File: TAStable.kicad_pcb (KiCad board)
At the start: 2 copper layers, 26.8 x 16.5 mm, 18 parts, among them J1 Conn_01x06_Pin, J2 ICSP, U1 74HCT1G04, U2 CS2300-CP, U3 74LVC1G14, U4 PIC16LF15313, U6 AZ1117-3.3

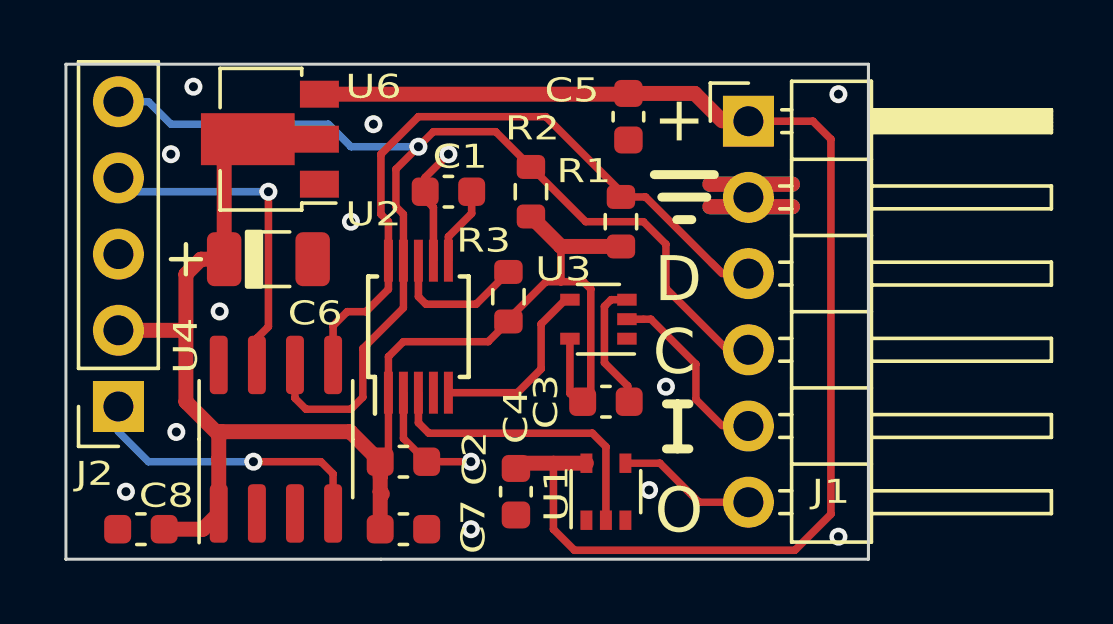
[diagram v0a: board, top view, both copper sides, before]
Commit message: more pics + cleanups
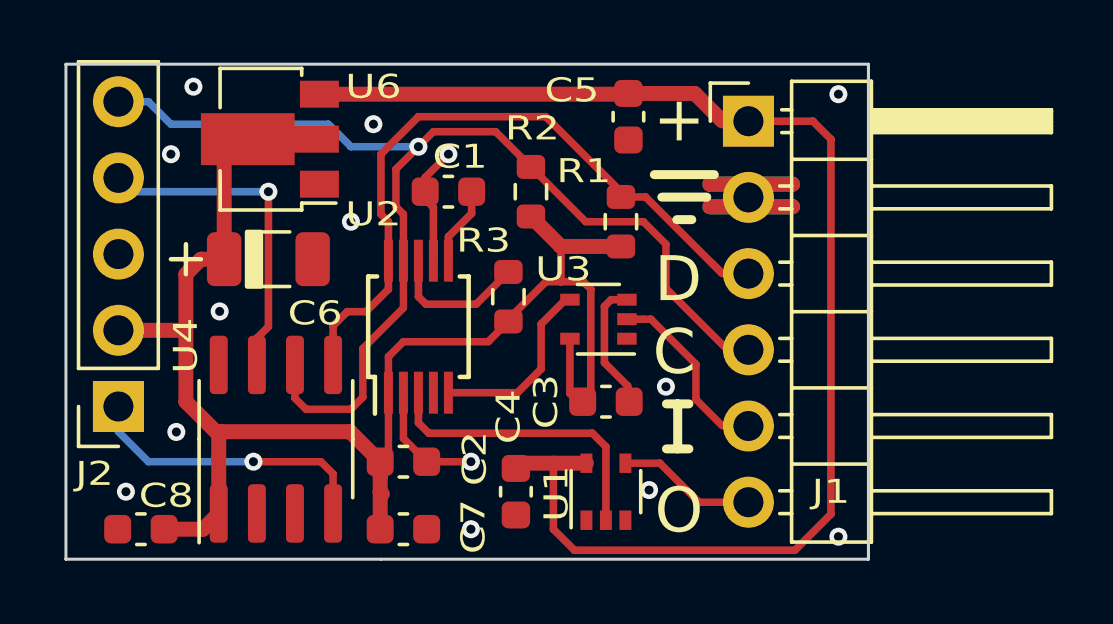
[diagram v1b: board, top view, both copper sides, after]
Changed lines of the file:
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@@
     (property "ki_keywords" "cap capacitor")
     (attr smd)
-    (fp_text reference "C4" (at -2.5 0 90) (layer "F.SilkS")
+    (fp_text reference "C4" (at -2.5 0.25 90) (layer "F.SilkS")
         (effects (font (size 0.8 1) (thickness 0.15)))
     )

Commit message: schematic
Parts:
- J1: value Conn_01x06_Pin -> IN/OUT
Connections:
- net Net-(J1-Pin_6) renamed /24MHz_OUT
- J1 pad 3: /I2C_SCL -> /I2C_SDA
- R1 pad 2: /I2C_SCL -> /I2C_SDA
- U2 pad 10: /I2C_SCL -> /I2C_SDA
- U4 pad 5: /I2C_SCL -> /I2C_SDA
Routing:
- net /I2C_SCL: track 61.8 -> 38.7 mm
- net /I2C_SDA: track 0.00 -> 23.1 mm
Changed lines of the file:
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@@
   (net 8 "/21MHz_IN")
   (net 9 "/I2C_SCL")
-  (net 10 "Net-(J1-Pin_6)")
+  (net 10 "/I2C_SDA")
   (net 11 "unconnected-(U4-RA5-Pad2)")
   (net 12 "unconnected-(U4-RA4-Pad3)")
@@
   (net 14 "/MCLR")
   (net 15 "/ICSPDAT")
+  (net 16 "/24MHz_OUT")
   (footprint "Package_SO:MSOP-10_3x3mm_P0.5mm" (layer "F.Cu")
     (at 130.25 100.5 90)
@@
       (net 9 "/I2C_SCL") (pinfunction "SCL/CCLK") (pintype "input"))
     (pad "10" smd rect (at 2.2 -1 90) (size 1.4 0.3) (layers "F.Cu" "F.Paste" "F.Mask")
-      (net 9 "/I2C_SCL") (pinfunction "SDA/CDIN") (pintype "bidirectional"))
+      (net 10 "/I2C_SDA") (pinfunction "SDA/CDIN") (pintype "bidirectional"))
     (model "${KICAD6_3DMODEL_DIR}/Package_SO.3dshapes/MSOP-10_3x3mm_P0.5mm.wrl"
       (offset (xyz 0 0 0))
@@
         (effects (font (size 0.8 1) (thickness 0.15)))
     )
-    (fp_text value "Conn_01x06_Pin" (at 1.865 16.18) (layer "F.Fab")
+    (fp_text value "IN/OUT" (at 1.865 16.18) (layer "F.Fab")
         (effects (font (size 0.8 1) (thickness 0.15)))
     )
@@
       (net 2 "GND") (pinfunction "Pin_2") (pintype "passive"))
     (pad "3" thru_hole oval (at 0 5.08) (size 1.7 1.7) (drill 1) (layers "*.Cu" "*.Mask")
-      (net 9 "/I2C_SCL") (pinfunction "Pin_3") (pintype "passive"))
+      (net 10 "/I2C_SDA") (pinfunction "Pin_3") (pintype "passive"))
     (pad "4" thru_hole oval (at 0 7.62) (size 1.7 1.7) (drill 1) (layers "*.Cu" "*.Mask")
       (net 9 "/I2C_SCL") (pinfunction "Pin_4") (pintype "passive"))
@@
       (net 8 "/21MHz_IN") (pinfunction "Pin_5") (pintype "passive"))
     (pad "6" thru_hole oval (at 0 12.7) (size 1.7 1.7) (drill 1) (layers "*.Cu" "*.Mask")
-      (net 10 "Net-(J1-Pin_6)") (pinfunction "Pin_6") (pintype "passive"))
+      (net 16 "/24MHz_OUT") (pinfunction "Pin_6") (pintype "passive"))
     (model "${KICAD6_3DMODEL_DIR}/Connector_PinHeader_2.54mm.3dshapes/PinHeader_1x06_P2.54mm_Horizontal.wrl"
       (offset (xyz 0 0 0))
@@
       (net 14 "/MCLR") (pinfunction "RA3") (pintype "input"))
     (pad "5" smd roundrect (at 2.475 1.905 90) (size 1.95 0.6) (layers "F.Cu" "F.Paste" "F.Mask") (roundrect_rratio 0.25)
-      (net 9 "/I2C_SCL") (pinfunction "RA2") (pintype "bidirectional"))
+      (net 10 "/I2C_SDA") (pinfunction "RA2") (pintype "bidirectional"))
     (pad "6" smd roundrect (at 2.475 0.635 90) (size 1.95 0.6) (layers "F.Cu" "F.Paste" "F.Mask") (roundrect_rratio 0.25)
       (net 9 "/I2C_SCL") (pinfunction "RA1") (pintype "bidirectional"))
@@
       (net 1 "+3.3V") (pintype "passive"))
     (pad "2" smd roundrect (at 0.825 0 90) (size 0.8 0.95) (layers "F.Cu" "F.Paste" "F.Mask") (roundrect_rratio 0.25)
-      (net 9 "/I2C_SCL") (pintype "passive"))
+      (net 10 "/I2C_SDA") (pintype "passive"))
     (model "${KICAD6_3DMODEL_DIR}/Resistor_SMD.3dshapes/R_0603_1608Metric.wrl"
       (offset (xyz 0 0 0))
@@
       (net 2 "GND") (pinfunction "GND") (pintype "power_in"))
     (pad "4" smd rect (at 0.95 0.65 90) (size 0.65 0.4) (layers "F.Cu" "F.Paste" "F.Mask")
-      (net 10 "Net-(J1-Pin_6)") (pintype "output"))
+      (net 16 "/24MHz_OUT") (pintype "output"))
     (pad "5" smd rect (at 0.95 -0.65 90) (size 0.65 0.4) (layers "F.Cu" "F.Paste" "F.Mask")
       (net 13 "+5V") (pinfunction "VCC") (pintype "power_in"))
@@
   (segment (start 138 100.25) (end 137.75 100.25) (width 0.25) (layer "F.Cu") (net 8))
   (segment (start 139.5 102.925) (end 139.5 101.75) (width 0.25) (layer "F.Cu") (net 8))
-  (segment (start 140.005 98.35) (end 140.375 98.72) (width 0.25) (layer "F.Cu") (net 9))
   (segment (start 129.75 98.3) (end 129.75 99.875) (width 0.25) (layer "F.Cu") (net 9))
   (segment (start 128 103.25) (end 126.5 103.25) (width 0.25) (layer "F.Cu") (net 9))
   (segment (start 130.25 94.5) (end 129.5 95.25) (width 0.25) (layer "F.Cu") (net 9))
-  (segment (start 130.25 93.5) (end 134.5 93.5) (width 0.254) (layer "F.Cu") (net 9))
   (segment (start 129.5 95.25) (end 129.5 96.5) (width 0.25) (layer "F.Cu") (net 9))
   (segment (start 140.54875 101.27) (end 141.25 101.27) (width 0.25) (layer "F.Cu") (net 9))
-  (segment (start 127.405 100.47) (end 127.875 100) (width 0.254) (layer "F.Cu") (net 9))
   (segment (start 138.5 97.75) (end 138.5 99.22125) (width 0.25) (layer "F.Cu") (net 9))
-  (segment (start 127.405 101.775) (end 127.405 100.47) (width 0.254) (layer "F.Cu") (net 9))
-  (segment (start 129 96.75) (end 129 94.75) (width 0.254) (layer "F.Cu") (net 9))
-  (segment (start 127.875 100) (end 128.5 100) (width 0.254) (layer "F.Cu") (net 9))
   (segment (start 126.135 102.885) (end 126.135 101.775) (width 0.25) (layer "F.Cu") (net 9))
   (segment (start 137.75 97) (end 138.5 97.75) (width 0.25) (layer "F.Cu") (net 9))
@@
   (segment (start 138.5 99.22125) (end 140.54875 101.27) (width 0.25) (layer "F.Cu") (net 9))
   (segment (start 129.5 96.5) (end 129.75 96.75) (width 0.25) (layer "F.Cu") (net 9))
-  (segment (start 129.25 97) (end 129 96.75) (width 0.254) (layer "F.Cu") (net 9))
-  (segment (start 129 94.75) (end 130.25 93.5) (width 0.254) (layer "F.Cu") (net 9))
-  (segment (start 129.25 99.25) (end 129.25 97) (width 0.254) (layer "F.Cu") (net 9))
   (segment (start 126.5 103.25) (end 126.135 102.885) (width 0.25) (layer "F.Cu") (net 9))
   (segment (start 129.75 99.875) (end 128.396838 101.228162) (width 0.25) (layer "F.Cu") (net 9))
-  (segment (start 134.5 93.5) (end 137.25 96.25) (width 0.254) (layer "F.Cu") (net 9))
-  (segment (start 140.375 98.73) (end 137.82 96.175) (width 0.254) (layer "F.Cu") (net 9))
-  (segment (start 137.82 96.175) (end 137 96.175) (width 0.254) (layer "F.Cu") (net 9))
   (segment (start 129.75 96.75) (end 129.75 98.3) (width 0.25) (layer "F.Cu") (net 9))
   (segment (start 130.75 94) (end 132.825 94) (width 0.25) (layer "F.Cu") (net 9))
-  (segment (start 128.5 100) (end 129.25 99.25) (width 0.254) (layer "F.Cu") (net 9))
   (via (at 130.25 94.5) (size 0.6) (drill 0.3) (layers "F.Cu" "B.Cu") (net 9))
   (segment (start 130.25 94.5) (end 128 94.5) (width 0.25) (layer "B.Cu") (net 9))
@@
   (segment (start 121.25 93) (end 120.25 93) (width 0.25) (layer "B.Cu") (net 9))
   (segment (start 128 94.5) (end 127.25 93.75) (width 0.25) (layer "B.Cu") (net 9))
-  (segment (start 141.25 106.35) (end 141.24 106.34) (width 0.254) (layer "F.Cu") (net 10))
-  (segment (start 137.15 105.05) (end 138.3 105.05) (width 0.25) (layer "F.Cu") (net 10))
-  (segment (start 138.3 105.05) (end 139.6 106.35) (width 0.25) (layer "F.Cu") (net 10))
-  (segment (start 139.6 106.35) (end 140.375 106.35) (width 0.25) (layer "F.Cu") (net 10))
+  (segment (start 140.005 98.35) (end 140.375 98.72) (width 0.25) (layer "F.Cu") (net 10))
+  (segment (start 130.25 93.5) (end 134.5 93.5) (width 0.254) (layer "F.Cu") (net 10))
+  (segment (start 127.405 100.47) (end 127.875 100) (width 0.254) (layer "F.Cu") (net 10))
+  (segment (start 127.405 101.775) (end 127.405 100.47) (width 0.254) (layer "F.Cu") (net 10))
+  (segment (start 129 96.75) (end 129 94.75) (width 0.254) (layer "F.Cu") (net 10))
+  (segment (start 127.875 100) (end 128.5 100) (width 0.254) (layer "F.Cu") (net 10))
+  (segment (start 129.25 97) (end 129 96.75) (width 0.254) (layer "F.Cu") (net 10))
+  (segment (start 129 94.75) (end 130.25 93.5) (width 0.254) (layer "F.Cu") (net 10))
+  (segment (start 129.25 99.25) (end 129.25 97) (width 0.254) (layer "F.Cu") (net 10))
+  (segment (start 134.5 93.5) (end 137.25 96.25) (width 0.254) (layer "F.Cu") (net 10))
+  (segment (start 140.375 98.73) (end 137.82 96.175) (width 0.254) (layer "F.Cu") (net 10))
+  (segment (start 137.82 96.175) (end 137 96.175) (width 0.254) (layer "F.Cu") (net 10))
+  (segment (start 128.5 100) (end 129.25 99.25) (width 0.254) (layer "F.Cu") (net 10))
   (segment (start 137.225 92.75) (end 126.95 92.75) (width 0.5) (layer "F.Cu") (net 13))
   (segment (start 139.46 92.725) (end 140.375 93.64) (width 0.5) (layer "F.Cu") (net 13))
@@
   (segment (start 125.25 96) (end 120.71 96) (width 0.254) (layer "B.Cu") (net 15))
   (segment (start 120.71 96) (end 120.25 95.54) (width 0.254) (layer "B.Cu") (net 15))
+  (segment (start 141.25 106.35) (end 141.24 106.34) (width 0.254) (layer "F.Cu") (net 16))
+  (segment (start 137.15 105.05) (end 138.3 105.05) (width 0.25) (layer "F.Cu") (net 16))
+  (segment (start 138.3 105.05) (end 139.6 106.35) (width 0.25) (layer "F.Cu") (net 16))
+  (segment (start 139.6 106.35) (end 140.375 106.35) (width 0.25) (layer "F.Cu") (net 16))
   (zone (net 2) (net_name "GND") (layers "F&B.Cu") (hatch edge 0.5)
     (connect_pads (clearance 0.5))
